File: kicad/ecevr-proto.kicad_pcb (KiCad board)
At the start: 4 copper layers, 86.3 x 69.7 mm, 222 parts, among them J19 SFP, J20 SFP_CAGE, J2001 IO_CONN, J2201 BEL_0845_2G1T_H5, J3 USB_C_Receptacle_USB2.0, J4 JTAG, J5 LSHM-150-04_JB1, J6 LSHM-150-04_JB2, Q1 SSM6N35AFE, Q2 SSM6N35AFE, Q3 Si3477, Q4 SSM6N35AFE, Q5 SSM6N35AFE, SW1 PROG, SW2101 SW_DIP_x08, U10 74LVC1G06, U12 5P49V6965, U13 TPS3808DBV, U14 74LVC1G06, U17 74LVC06, U18 74LVC1T126, U2001 74LVC2T45DC, U21 74LVC1G06, U2101 74AHC1T86, U2102 74AHC1T86, U2103 PCA9306, U2104 24FC16T, U2105 74AHC1T86, U2106 74AHC1T86, U2201 74AHC1T86, U2202 74LVC1G06, U2301 lan9254, U8 74ALVC125, U9 TLV62569ADDC, X2301 FNETHE025, Y1 25MHz

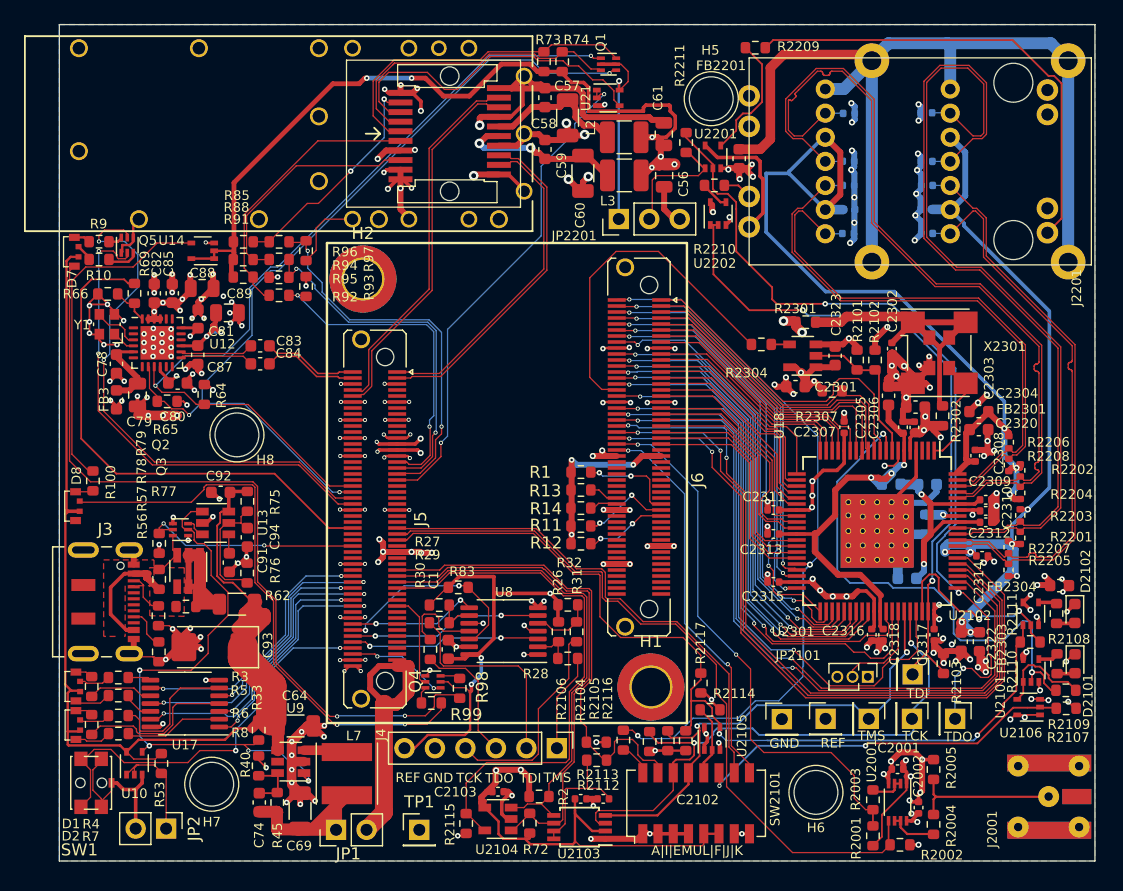
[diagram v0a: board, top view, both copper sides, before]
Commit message: prepared for JLCPCB; created gerbers
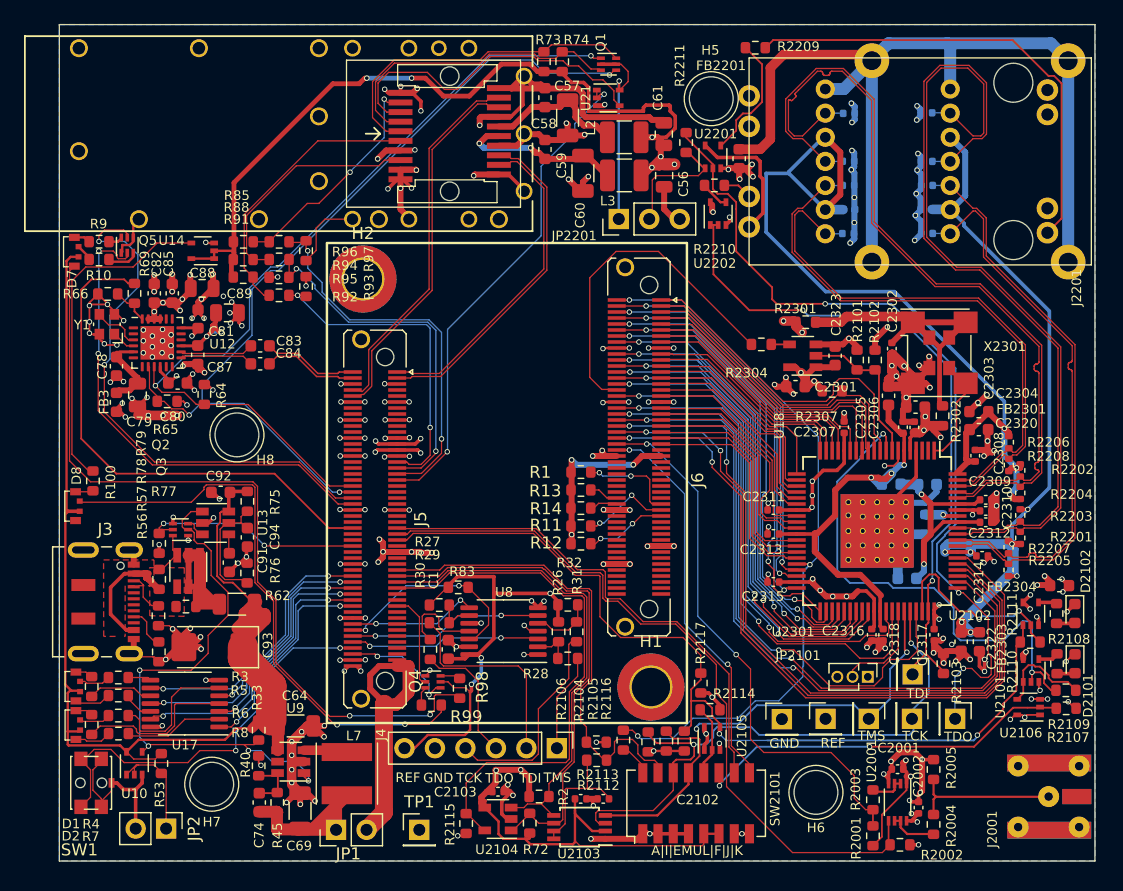
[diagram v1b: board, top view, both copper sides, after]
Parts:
- moved C78 0.20 mm to (118.5, 58.3)
- moved FB3 0.20 mm to (118.5, 61.3)
- moved R99 0.17 mm to (144.7, 86.5)
- moved R2105 0.12 mm to (164.3, 89.5)
- moved R2116 0.12 mm to (165.8, 89.5)
- moved R2104 0.12 mm to (162.8, 89.6)
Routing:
- net IO_L24N_34: track 19.6 -> 17.7 mm
- net IO_L20N_34: track 19.5 -> 17.6 mm
- net IO_L18P_34: track 18.9 -> 17.1 mm
- net /SFP Connector/TX_DISABLE: track 27.1 -> 28.2 mm
- net /CFG_DONE: track 8.47 -> 9.53 mm
- net IO_L18N_34: track 23.1 -> 23.8 mm
- net GND: vias 213 -> 212
- net +3V3: track 206.4 -> 206.3 mm, vias 25 -> 24
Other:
- rule pad_to_mask_clearance: 0.048 -> 0
